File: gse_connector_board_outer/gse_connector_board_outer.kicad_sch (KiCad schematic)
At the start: 8 parts, among them J1 arming_connector, J2 gse_com_connector, J3 chg_connector, J5 Conn_02x02_Top_Bottom, J6 Conn_02x02_Top_Bottom, J7 Conn_02x02_Top_Bottom

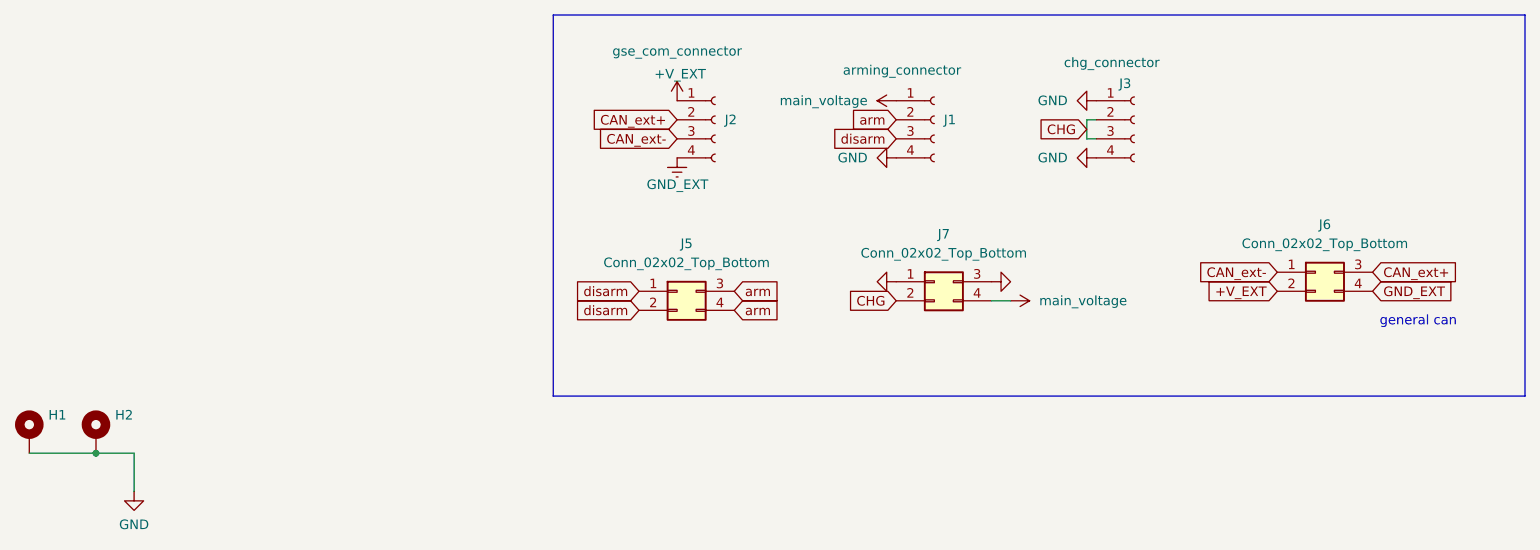
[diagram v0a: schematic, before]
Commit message: implemented changes
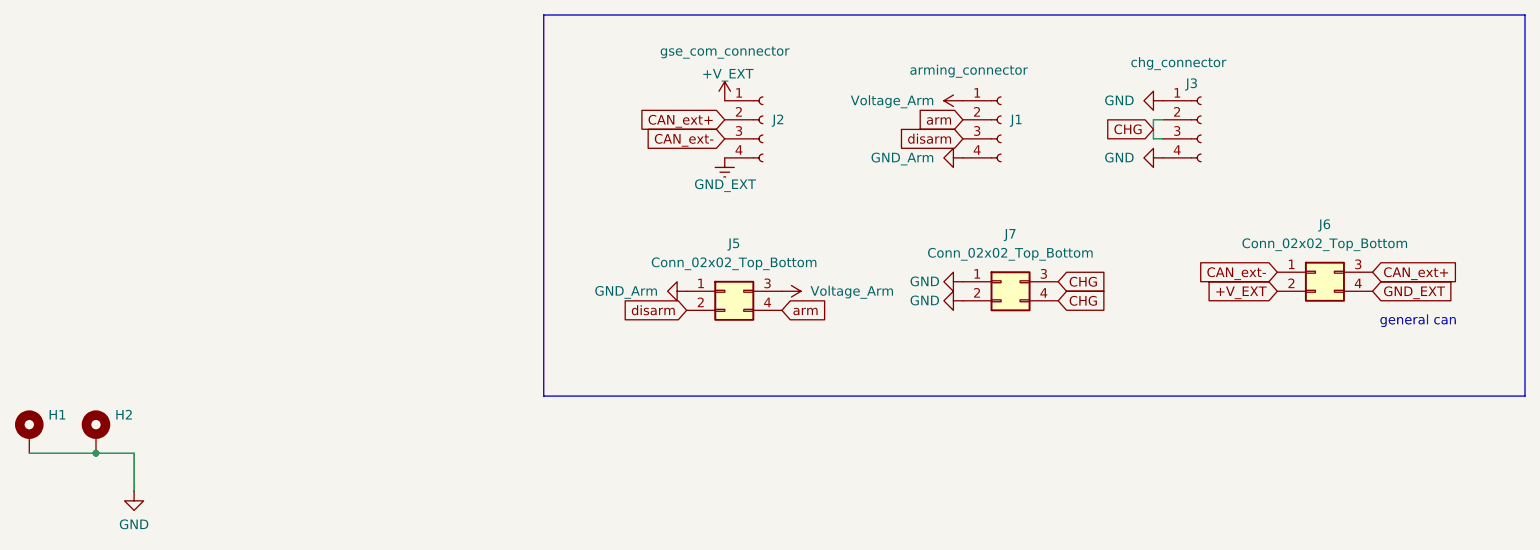
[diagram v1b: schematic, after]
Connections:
- net CHG: now also J7.3 (Pin_3), J7.4 (Pin_4); no longer J7.2 (Pin_2)
- net GND: now also J7.2 (Pin_2); no longer J1.4 (Pin_4), J7.3 (Pin_3)
- net arm: no longer J5.3 (Pin_3)
- net disarm: no longer J5.1 (Pin_1)
- net main_voltage renamed Voltage_Arm
- net Voltage_Arm: now also J5.3 (Pin_3); no longer J7.4 (Pin_4)
- new net GND_Arm: J1.4 (Pin_4), J5.1 (Pin_1)
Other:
- moved on the sheet: J1, J2, J3, J5, J7
